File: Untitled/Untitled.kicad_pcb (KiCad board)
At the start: 4 copper layers, 55 x 40 mm, 67 parts, among them J1 Conn_02x07_Top_Bottom, J2 USB4125-GF-A-0190, J3 Screw_Terminal_01x02, U1 STM32F070CBT6TR, U2 INA180A1, U3 SPX3819M5-L-3-3, U4 SPX3819M5-L-3-3, U5 TPS7A0522PDBZT, U6 AL5809-20QP1-7, U7 MCP6L01x-xLT, U8 AP331AWG-7, Y1 ABM8G-12.000MHZ-18-D2Y-T

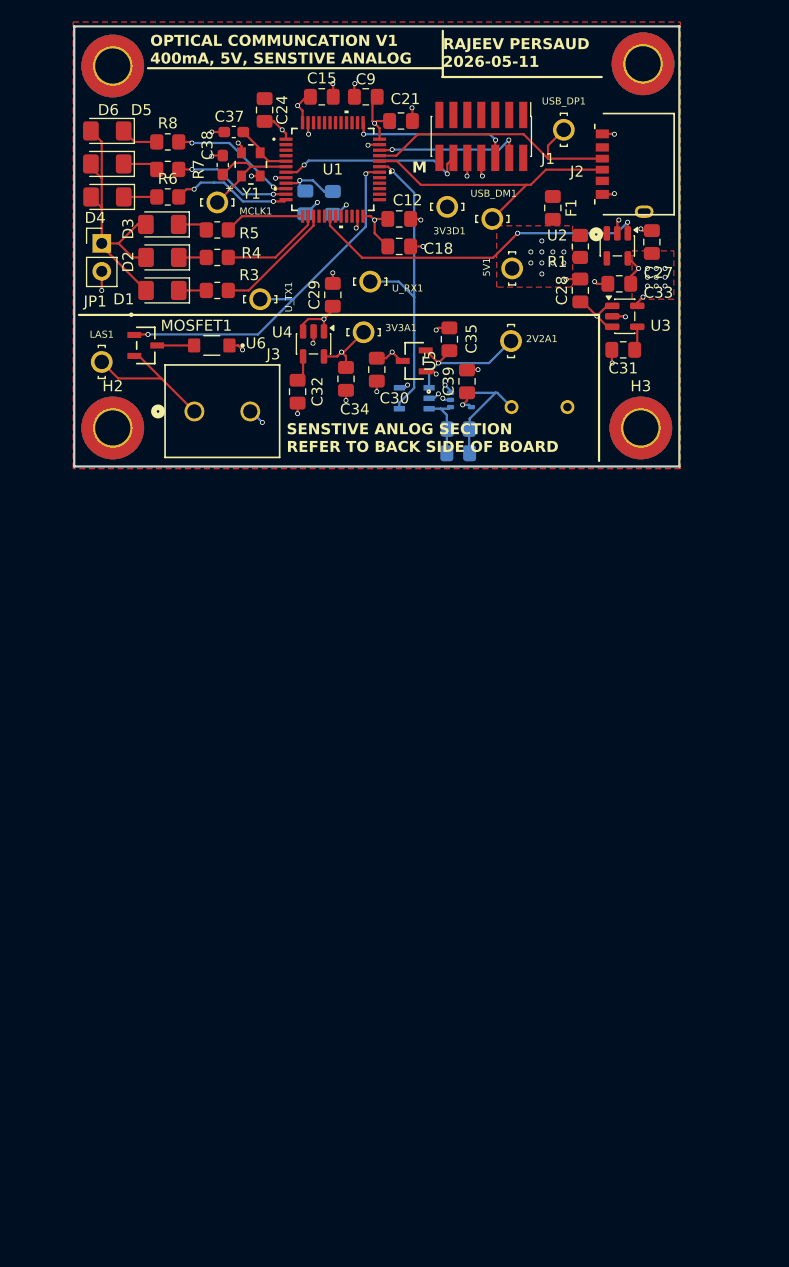
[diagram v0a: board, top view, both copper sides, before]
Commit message: revised verison
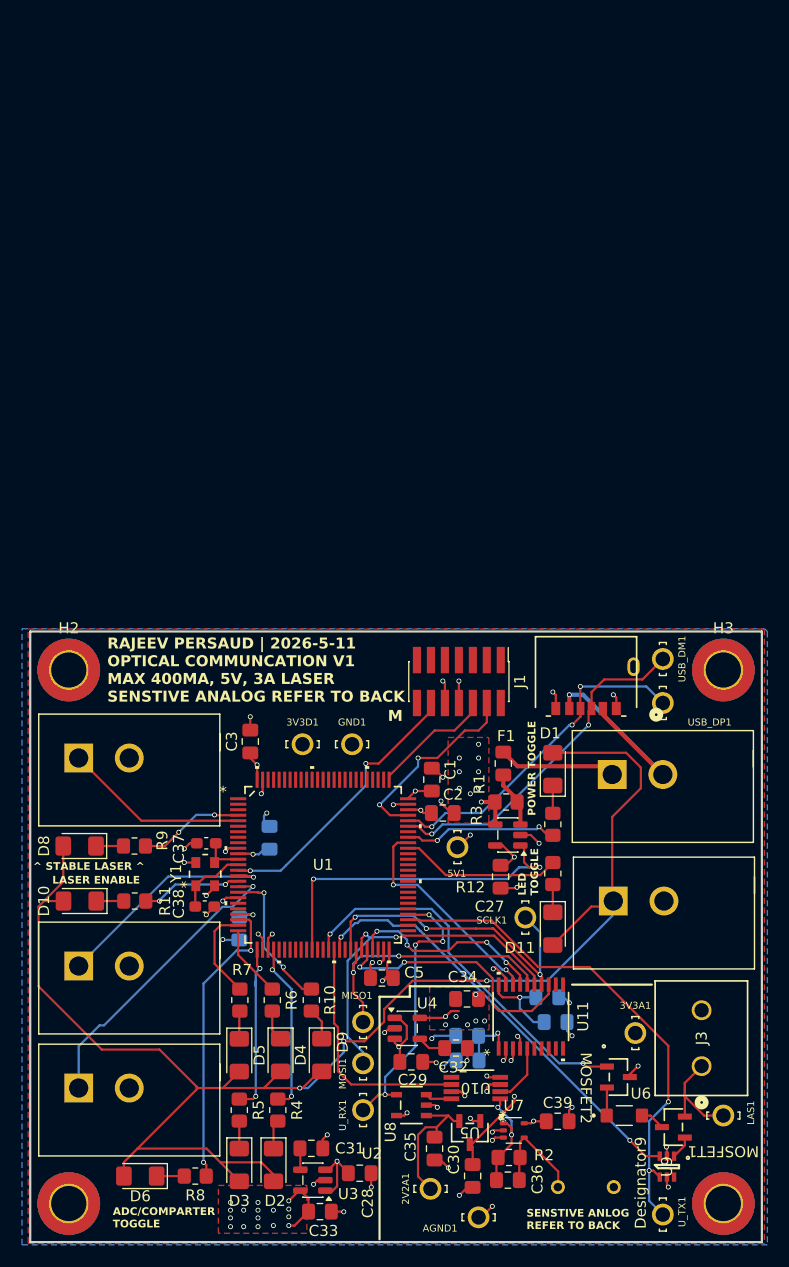
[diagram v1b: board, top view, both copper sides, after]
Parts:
- removed C12, C15, C18, C21, C24: 0.1uF, Capacitor_SMD:C_0805_2012Metric_Pad1.18x1.45mm_HandSolder
- removed the G*** at (43.4, 41.2)
- removed the G*** at (27.4, 64.2)
- removed JP1: Jumper_2_Bridged, Connector_PinHeader_2.54mm:PinHeader_1x02_P2.54mm_Vertical
- removed MCLK1: 4952, USB-c:KEYSTONE_4952
- added AGND1: 4952, USB-c:KEYSTONE_4952, F.Cu at (53.2, 143.2)
- added C10: 1uF, Capacitor_SMD:C_0805_2012Metric_Pad1.18x1.45mm_HandSolder, B.Cu at (31.5, 117.0)
- added C2: 1uF, Capacitor_SMD:C_0805_2012Metric_Pad1.18x1.45mm_HandSolder, F.Cu at (50.0, 106.5)
- added C4: 1uF, Capacitor_SMD:C_0805_2012Metric_Pad1.18x1.45mm_HandSolder, B.Cu at (34.2, 108.8)
- added C5: 1uF, Capacitor_SMD:C_0805_2012Metric_Pad1.18x1.45mm_HandSolder, F.Cu at (44.5, 121.5)
- added C6: 0.1uF, Capacitor_SMD:C_0805_2012Metric_Pad1.18x1.45mm_HandSolder, B.Cu at (52.2, 126.8)
- added C7: 10uF, Capacitor_SMD:C_0805_2012Metric_Pad1.18x1.45mm_HandSolder, B.Cu at (52.2, 129.0)
- added C8: 0.1uF, Capacitor_SMD:C_0805_2012Metric_Pad1.18x1.45mm_HandSolder, B.Cu at (60.2, 125.5)
- added D10: GREEN LED, LED_SMD:LED_1206_3216Metric_Pad1.42x1.75mm_HandSolder, F.Cu at (17.0, 114.5)
- added D11: GREEN LED, LED_SMD:LED_1206_3216Metric_Pad1.42x1.75mm_HandSolder, F.Cu at (60.0, 117.0)
- added D8: RED LED, LED_SMD:LED_1206_3216Metric_Pad1.42x1.75mm_HandSolder, F.Cu at (17.0, 109.5)
- added D9: GREEN LED, LED_SMD:LED_1206_3216Metric_Pad1.42x1.75mm_HandSolder, F.Cu at (39.0, 128.5)
- added G***: LOGO, LOGO, B.Cu at (41.8, 98.8)
- added G***: LOGO, LOGO, B.Cu at (33.0, 135.0)
- added GND1: 4952, USB-c:KEYSTONE_4952, F.Cu at (41.8, 100.2)
- added MISO1: 4952, USB-c:KEYSTONE_4952, F.Cu at (42.8, 125.5)
- added MOSFET2: 2N7002, USB-c:SOT-23TO-236_318-08_ONS, F.Cu at (66.0, 130.5)
- added MOSI1: 4952, USB-c:KEYSTONE_4952, F.Cu at (42.8, 129.2)
- added R10: 220R, Resistor_SMD:R_0805_2012Metric_Pad1.20x1.40mm_HandSolder, F.Cu at (38.0, 123.5)
- added R11: 220R, Resistor_SMD:R_0805_2012Metric_Pad1.20x1.40mm_HandSolder, F.Cu at (22.0, 114.5)
- added R12: 220R, Resistor_SMD:R_0805_2012Metric_Pad1.20x1.40mm_HandSolder, F.Cu at (60.0, 112.0)
- added R9: 220R, Resistor_SMD:R_0805_2012Metric_Pad1.20x1.40mm_HandSolder, F.Cu at (22.0, 109.5)
- added S1: GF-123-0054, USB-c:SW_GF-123-0054, F.Cu at (70.0, 104.1)
- added S2: GF-123-0054, USB-c:SW_GF-123-0054, F.Cu at (21.5, 102.6)
- added S3: GF-123-0054, USB-c:SW_GF-123-0054, F.Cu at (21.5, 132.6)
- added S4: GF-123-0054, USB-c:SW_GF-123-0054, F.Cu at (21.5, 121.5)
- added S5: GF-123-0054, USB-c:SW_GF-123-0054, F.Cu at (70.1, 115.6)
- added SCLK1: 4952, USB-c:KEYSTONE_4952, F.Cu at (57.5, 116.0)
- added U10: ADG1419BRMZ, USB-c:RM_8_ADI, F.Cu at (53.0, 131.5)
- added U11: MCP3462-E/ST, USB-c:TSSOP20_ST_MCH_MIS, F.Cu at (58.0, 125.0)
- added U9: SN74LVC1G332DCKR, USB-c:DCK0006A_N, F.Cu at (70.4, 138.6)
- C1, C36, R2, U7, U8: moved to F.Cu
- C3: value 10nF -> 1uF; moved to F.Cu
- C9: value 4.7uF -> 10uF; moved to B.Cu
- J1: value Conn_02x07_Top_Bottom -> Debugging Connector
- U1: value STM32F070CBT6TR -> STM32H523VET6; footprint USB-c:LQFP48-7x7mm -> USB-c:LQFP-100
- moved H4 103.9 mm to (75.5, 142.0)
- moved H1 103.5 mm to (16.0, 142.0)
- moved D6 95.0 mm to (22.5, 139.5)
- moved R8 94.0 mm to (27.5, 139.5)
- moved U_TX1 90.9 mm to (70.0, 143.0), turned to -90 degrees
- moved LAS1 88.8 mm to (75.5, 134.0), turned to 0 degrees
- moved C33 88.6 mm to (38.8, 142.7), turned to 0 degrees
- moved D3 85.8 mm to (31.5, 138.5), turned to -90 degrees
- moved MOSFET1 85.7 mm to (71.0, 135.0), turned to 90 degrees
- moved C9 83.5 mm to (59.5, 123.2), turned to 0 degrees
- moved U3 83.5 mm to (38.2, 139.9), turned to 180 degrees
- moved D2 83.1 mm to (34.6, 138.5), turned to -90 degrees
- moved C28 82.7 mm to (42.4, 139.2), turned to 0 degrees
- moved D5 81.9 mm to (31.5, 128.5), turned to -90 degrees
- moved R5 80.0 mm to (31.5, 133.5), turned to 90 degrees
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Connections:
- net Net-(D1-A) renamed /MCU/ADC_LED
- C1 pad 1: +3.3VA -> GND
- C1 pad 2: GND -> +3.3VD
- C3 pad 1: +3.3VA -> +3.3VD
- C36 pad 2: Net-(U8-IN+) -> Net-(U10-D)
- C39 pad 1: +3.3VD -> +5V
- J2 pad 2: Net-(F1-Pad1) -> Net-(J2-Pad2)
- J2 pad 5: Net-(F1-Pad1) -> Net-(J2-Pad2)
- MOSFET1 pad 1: /Laser/UART_TX -> Net-(MOSFET1-G)
- R2 pad 2: Net-(U8-IN+) -> Net-(U10-D)
- R3 pad 2: Net-(U1A-PA5) -> Net-(U1A-PA9)
- U1 pad 1: +3.3VD -> unconnected-(U1B-PE2-Pad1)
- U1 pad 10: Net-(U1A-PA0) -> GND
- U1 pad 11: Net-(U1A-PA1) -> +3.3VD
- U1 pad 12: Net-(U1A-PA2) -> /MCU/MCLCK_IN
- U1 pad 13: Net-(U1A-PA3) -> /MCU/MCLCK_OUT
- U1 pad 14: Net-(U1A-PA4) -> /MCU/MCLR
- U1 pad 15: Net-(U1A-PA5) -> /MCU/HARD_LAS_ENB
- U1 pad 16: unconnected-(U1A-PA6-Pad16) -> Net-(U1A-PC1)
- U1 pad 17: unconnected-(U1A-PA7-Pad17) -> /MCU/HARD_ADC_COMP
- U1 pad 18: /MCU/CUR_SEN -> Net-(U1A-PC3)
- U1 pad 19: unconnected-(U1A-PB1-Pad19) -> GND
- U1 pad 22: unconnected-(U1A-PB11-Pad22) -> +3.3VD
- U1 pad 23: GND -> Net-(U1A-PA0)
- U1 pad 24: +3.3VD -> Net-(U1A-PA1)
- U1 pad 25: unconnected-(U1A-PB12-Pad25) -> Net-(U1A-PA2)
- U1 pad 26: unconnected-(U1A-PB13-Pad26) -> Net-(U1A-PA3)
- U1 pad 27: unconnected-(U1A-PB14-Pad27) -> GND
- U1 pad 28: unconnected-(U1A-PB15-Pad28) -> +3.3VD
- U1 pad 29: unconnected-(U1A-PA8-Pad29) -> Net-(U1A-PA4)
- U1 pad 30: /Laser/UART_TX -> unconnected-(U1A-PA5-Pad30)
- U1 pad 31: /Analog Amplifer/UART_RX -> unconnected-(U1A-PA6-Pad31)
- U1 pad 32: /MCU/USB_DM -> unconnected-(U1A-PA7-Pad32)
- U1 pad 33: /MCU/USB_DP -> unconnected-(U1A-PC4-Pad33)
- U1 pad 34: /MCU/PGC -> unconnected-(U1A-PC5-Pad34)
- U1 pad 35: GND -> unconnected-(U1A-PB0-Pad35)
- U1 pad 36: +3.3VD -> /MCU/CUR_SEN
- U1 pad 37: /MCU/PGD -> unconnected-(U1A-PB2-Pad37)
- U1 pad 39: unconnected-(U1A-PB3-Pad39) -> /PIN_LAS_ENB
- U1 pad 4: unconnected-(U1A-PC15-OSC32_OUT-Pad4) -> Net-(U1B-PE5)
- U1 pad 40: unconnected-(U1A-PB4-Pad40) -> /PIN_SWAP_ADC
- U1 pad 41: unconnected-(U1A-PB5-Pad41) -> /PIN_BYPASS_MOSFET
- U1 pad 43: unconnected-(U1A-PB7-Pad43) -> /SCLK
- U1 pad 44: unconnected-(U1A-BOOT0-Pad44) -> /MISO
- U1 pad 45: unconnected-(U1A-PB8-Pad45) -> /MOSI
- U1 pad 46: unconnected-(U1A-PB9-Pad46) -> /CS_ADC
- U1 pad 47: GND -> /IRQ
- U1 pad 48: +3.3VD -> unconnected-(U1B-VCAP-Pad48)
- U1 pad 5: /MCU/MCLCK_IN -> /MCU/HARD_BYPASS_MOSFET
- U1 pad 6: /MCU/MCLCK_OUT -> unconnected-(U1B-VBAT-Pad6)
- U1 pad 7: /MCU/MCLR -> unconnected-(U1A-PC13-Pad7)
- U1 pad 8: GND -> unconnected-(U1A-PC14-OSC32_IN-Pad8)
- U1 pad 9: +3.3VA -> unconnected-(U1A-PC15-OSC32_OUT-Pad9)
- U6 pad 1: +3.3VA -> Net-(MOSFET2-S)
- U7 pad 1: Net-(U8-IN+) -> Net-(U10-D)
- U7 pad 5: +3.3VD -> +5V
- U8 pad 3: Net-(U8-IN+) -> Net-(U10-SB)
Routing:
- net /MCU/ADC_LED: track 27.4 -> 143.0 mm, vias 0 -> 3
- net /PIN_BYPASS_MOSFET: track 0.00 -> 39.7 mm, vias 0 -> 2
- net /PIN_LAS_ENB: track 0.00 -> 34.9 mm, vias 0 -> 2
- net /MOSI: track 0.00 -> 32.3 mm, vias 0 -> 2
- net /SCLK: track 0.00 -> 28.9 mm, vias 0 -> 3
- net /MCU/HARD_ADC_COMP: track 0.00 -> 27.0 mm, vias 0 -> 1
- net /MISO: track 0.00 -> 25.5 mm, vias 0 -> 2
- net /CS_ADC: track 0.00 -> 24.1 mm, vias 0 -> 2
- net GND: track 40.8 -> 64.6 mm, vias 36 -> 47
- net /PIN_SWAP_ADC: track 0.00 -> 22.0 mm
- net Net-(J2-Pad2): track 0.00 -> 21.0 mm, vias 0 -> 1
- net /MCU/HARD_LAS_ENB: track 0.00 -> 20.7 mm, vias 0 -> 1
- net /REF_CLK: track 0.00 -> 20.0 mm, vias 0 -> 2
- net /IRQ: track 0.00 -> 18.3 mm, vias 0 -> 4
- net /MCU/HARD_BYPASS_MOSFET: track 0.00 -> 16.9 mm
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- added copper zone on F.Cu, net +3.3VA
- added copper zone on B.Cu, net GND
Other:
- board size 55 x 40 mm -> 66.5 x 55.5 mm
- board text added: "<-"
- board text added: "ADC/COMPARTER TOGGLE"
- board text added: "LASER ENABLE"
- board text added: "LED TOGGLE"
- board text added: "POWER TOGGLE"
- board text added: "RAJEEV PERSAUD | 2026-5-11 OPTICAL COMMUNCATION V1 MAX 400MA, 5V, 3A LASER SENSTIVE ANALOG REFER TO BACK"
- board text added: "SENSTIVE ANLOG REFER TO BACK"
- board text added: "SENSTIVE PHOTODIODE & AMPLIFER DO NOT TOUCH WITHOUT GLOVES ADVOID NEARBY EMI"
- board text added: "^ STABLE LASER ^"
- board text removed: "OPTICAL COMMUNCATION V1 400mA, 5V, SENSTIVE ANALOG"
- board text removed: "RAJEEV PERSAUD 2026-05-11"
- board text removed: "SENSTIVE ANLOG SECTION REFER TO BACK SIDE OF BOARD"
- board text removed: "SENSTIVE PHOTODIODE & AMPLIFER USE GLOVES | ADVOID EMI"
